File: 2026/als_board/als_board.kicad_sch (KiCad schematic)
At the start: 18 parts, among them J1 MAIN, J2 i2c, J3 PROG, U1 GM7333, U2 ME6209A50M3G, U3 CH32V003JxMx, U4 MAX485E

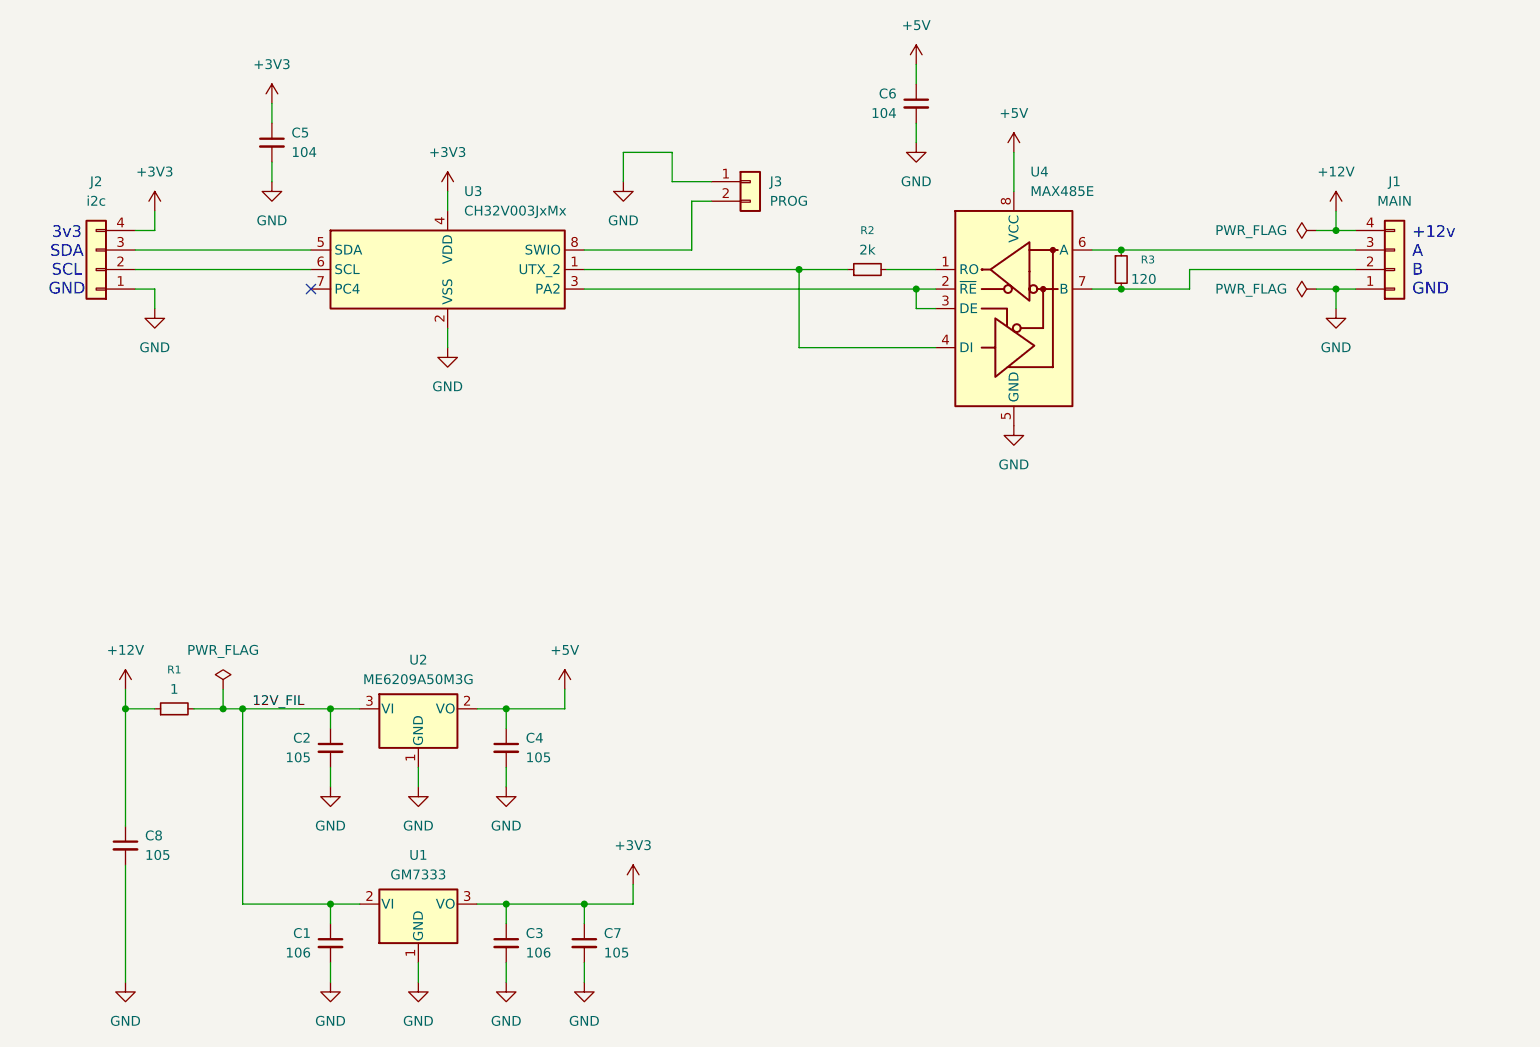
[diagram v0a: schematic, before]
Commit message: ALS finishing touches
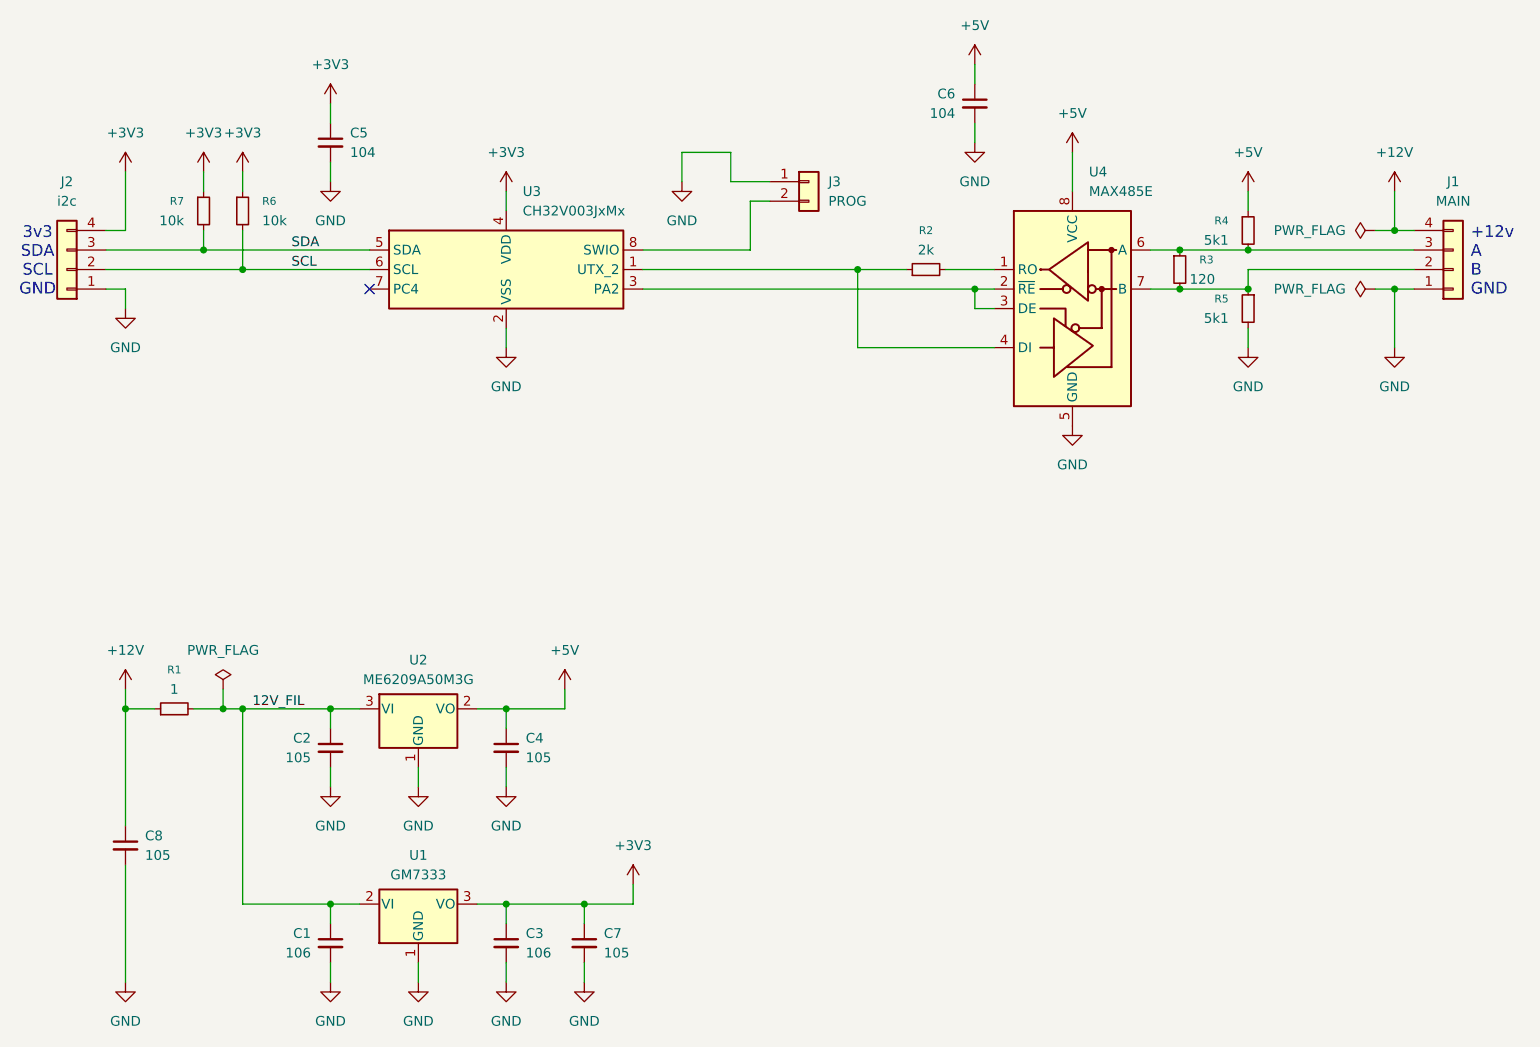
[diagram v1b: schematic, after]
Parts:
- added R4, R5: 5k1, Resistor_SMD:R_0603_1608Metric, symbol Device:R_Small
- added R6, R7: 10k, Resistor_SMD:R_0603_1608Metric, symbol Device:R_Small
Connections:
- net +3V3: now also R6.1, R7.1
- net +5V: now also R4.1
- net GND: now also R5.2
- net SCL: now reaches J2.2 (Pin_2), U3.6 (PC2)
- net SCL: now also R6.2
- net SDA: now reaches J2.3 (Pin_3), U3.5 (PC1)
- net SDA: now also R7.2
- net at J1.3 (Pin_3), R3.1, U4.6 (A): now also R4.2
- net at J1.2 (Pin_2), R3.2, U4.7 (B): now also R5.1
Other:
- moved on the sheet: C5, C6, J1, J2, J3, R2, R3, U3, U4
